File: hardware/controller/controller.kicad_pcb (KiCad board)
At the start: 2 copper layers, 47 parts, among them J1 Conn_01x02_Pin, J11 Barrel_Jack, J12 USB_C_Receptacle_USB2.0_14P, J2 Conn_01x02_Pin, J3 Conn_01x02_Pin, J5 Screw_Terminal_01x02, J6 Screw_Terminal_01x02, J7 Conn_01x04_Pin, J8 Conn_01x04_Pin, U1 ESP32-C3-MINI-1, U2 MAX31855KASA, U3 MAX31855KASA, U4 MAX31855KASA, U6 TPS1H200AQDGNRQ1, U7 MPM3606AGQV-P, U8 LM73100RPWR, U9 LM73100RPWR

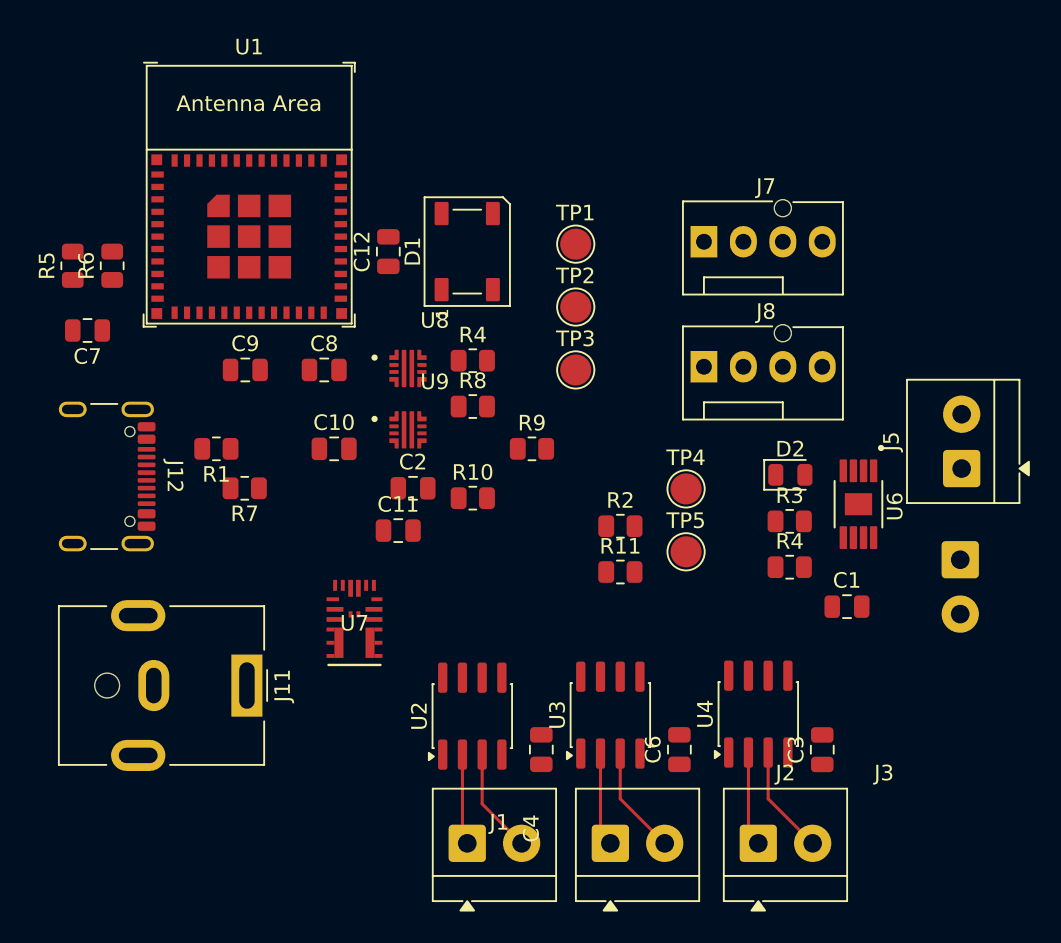
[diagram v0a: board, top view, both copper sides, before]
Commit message: First stab at board routing
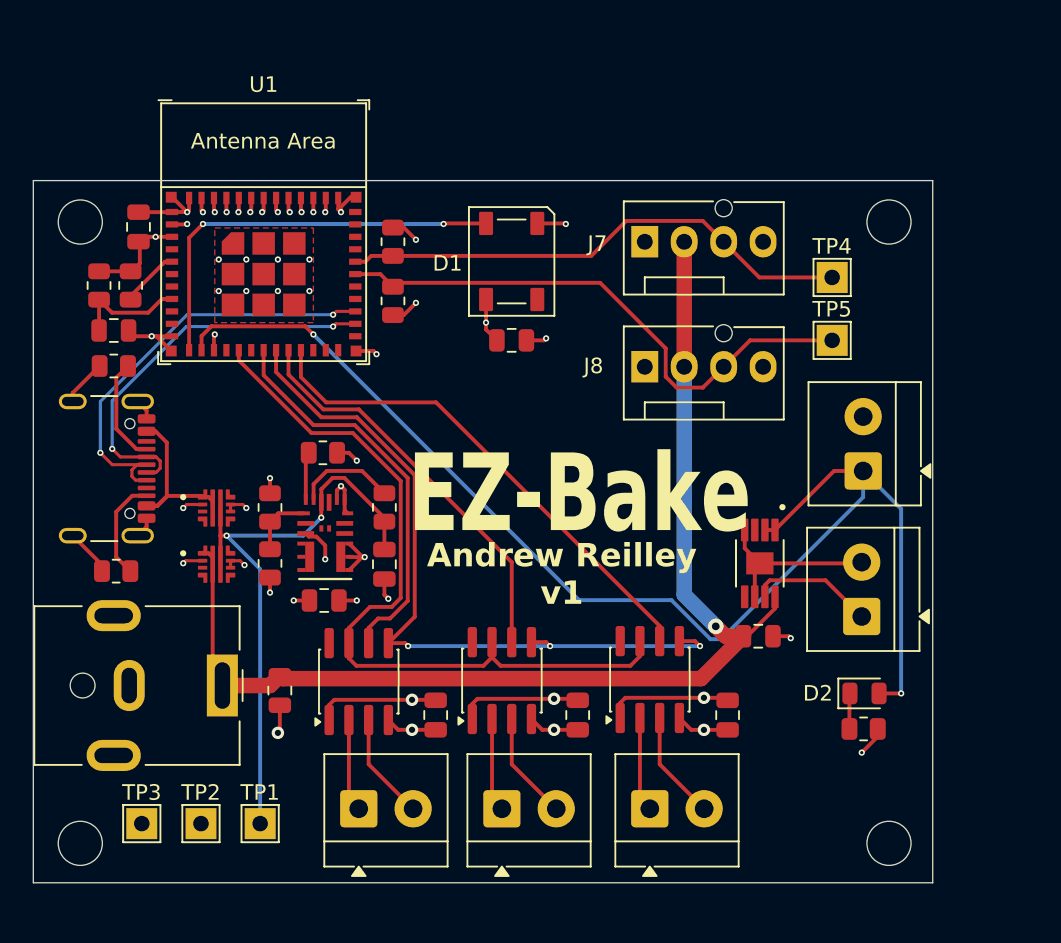
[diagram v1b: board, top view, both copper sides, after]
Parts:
- removed C9: 0.1uf, Capacitor_SMD:C_0805_2012Metric
- removed the R4 at (155.4, 96.5)
- J6: moved to F.Cu
- TP1, TP2, TP3, TP4, TP5: footprint TestPoint:TestPoint_Pad_D2.0mm -> TestPoint:TestPoint_THTPad_2.0x2.0mm_Drill1.0mm
- moved TP1 42.5 mm to (121.3, 113.0)
- moved TP2 41.1 mm to (117.5, 113.0)
- moved TP3 40.4 mm to (113.7, 113.0)
- moved R2 23.4 mm to (129.8, 75.6), turned to 90 degrees
- moved R11 22.8 mm to (129.8, 79.4), turned to -90 degrees
- moved R9 18.4 mm to (121.9, 96.3), turned to -90 degrees
- moved TP4 16.5 mm to (158.1, 77.9)
- moved TP5 16.5 mm to (158.1, 81.9)
- moved C2 15.6 mm to (122.6, 104.5), turned to -90 degrees
- moved U8 15.3 mm to (118.5, 92.7)
- moved C8 15.1 mm to (113.5, 74.6), turned to 90 degrees
- moved U9 15.1 mm to (118.5, 96.3)
- moved D2 14.9 mm to (160.2, 104.6)
- moved R8 14.6 mm to (121.9, 92.7), turned to -90 degrees
- moved R3 14.2 mm to (160.1, 106.9)
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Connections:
- U1 pad 18: SCK -> CS0
- U1 pad 19: CS0 -> SCK
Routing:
- net GND: track 0.00 -> 95.5 mm, vias 0 -> 43
- net /Microcontroller/HEATER: track 0.00 -> 82.3 mm, vias 0 -> 2
- net +12V: track 0.00 -> 75.5 mm, vias 0 -> 1
- net SO: track 0.00 -> 49.9 mm
- net SCK: track 0.00 -> 47.5 mm, vias 0 -> 3
- net VBUS: track 0.00 -> 39.3 mm, vias 0 -> 2
- net FAN_1_TACH: track 0.00 -> 36.3 mm
- net FAN_0_TACH: track 0.00 -> 33.3 mm
- net CS2: track 0.00 -> 32.4 mm
- net +3V3: track 0.00 -> 28.7 mm, vias 0 -> 10
- net /Microcontroller/USB_D+: track 0.00 -> 28.0 mm, vias 0 -> 2
- net /Microcontroller/LED: track 0.00 -> 26.7 mm, vias 0 -> 2
- net CS1: track 0.00 -> 26.1 mm
- net CS0: track 0.00 -> 25.8 mm
- net /Microcontroller/USB_D-: track 0.00 -> 25.7 mm, vias 0 -> 2
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- added copper zone on In2.Cu, net +3V3
- added copper zone on F.Cu, net GND
- added copper zone on In1.Cu, net GND
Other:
- board outline added: 57.9 x 45.2 mm
- copper layers 2 -> 4
- board text added: "Andrew Reilley v1"
- board text added: "EZ-Bake"
